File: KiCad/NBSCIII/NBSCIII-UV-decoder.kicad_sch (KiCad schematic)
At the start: 29 parts, among them U2 4053, U3 LM324N

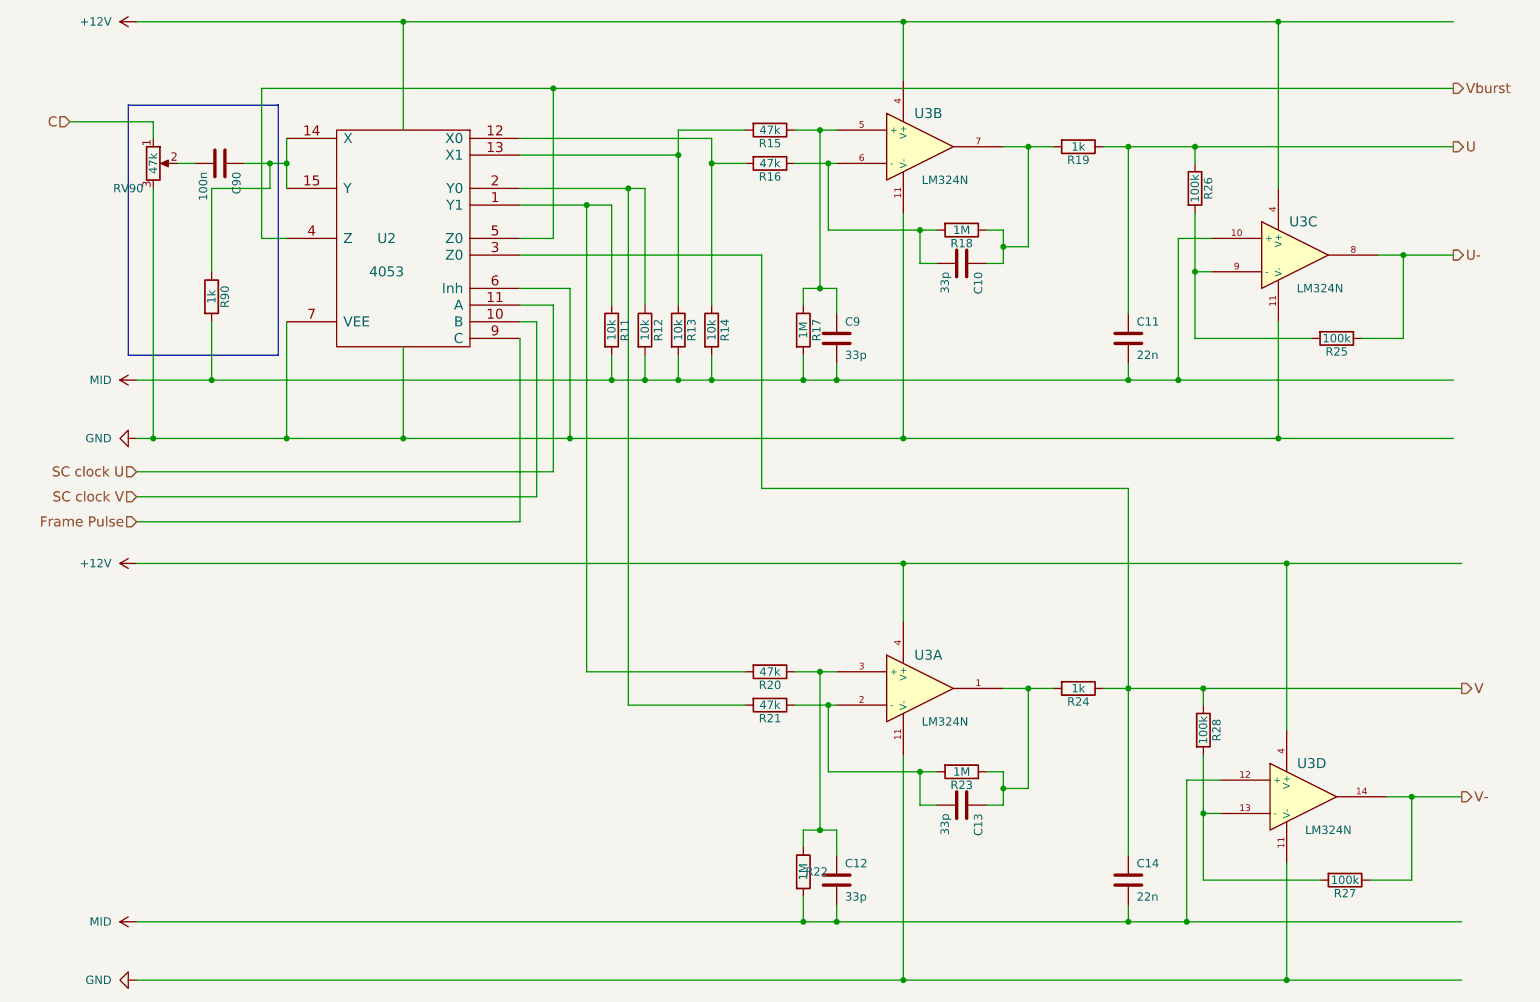
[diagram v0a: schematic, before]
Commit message: derescue 4053
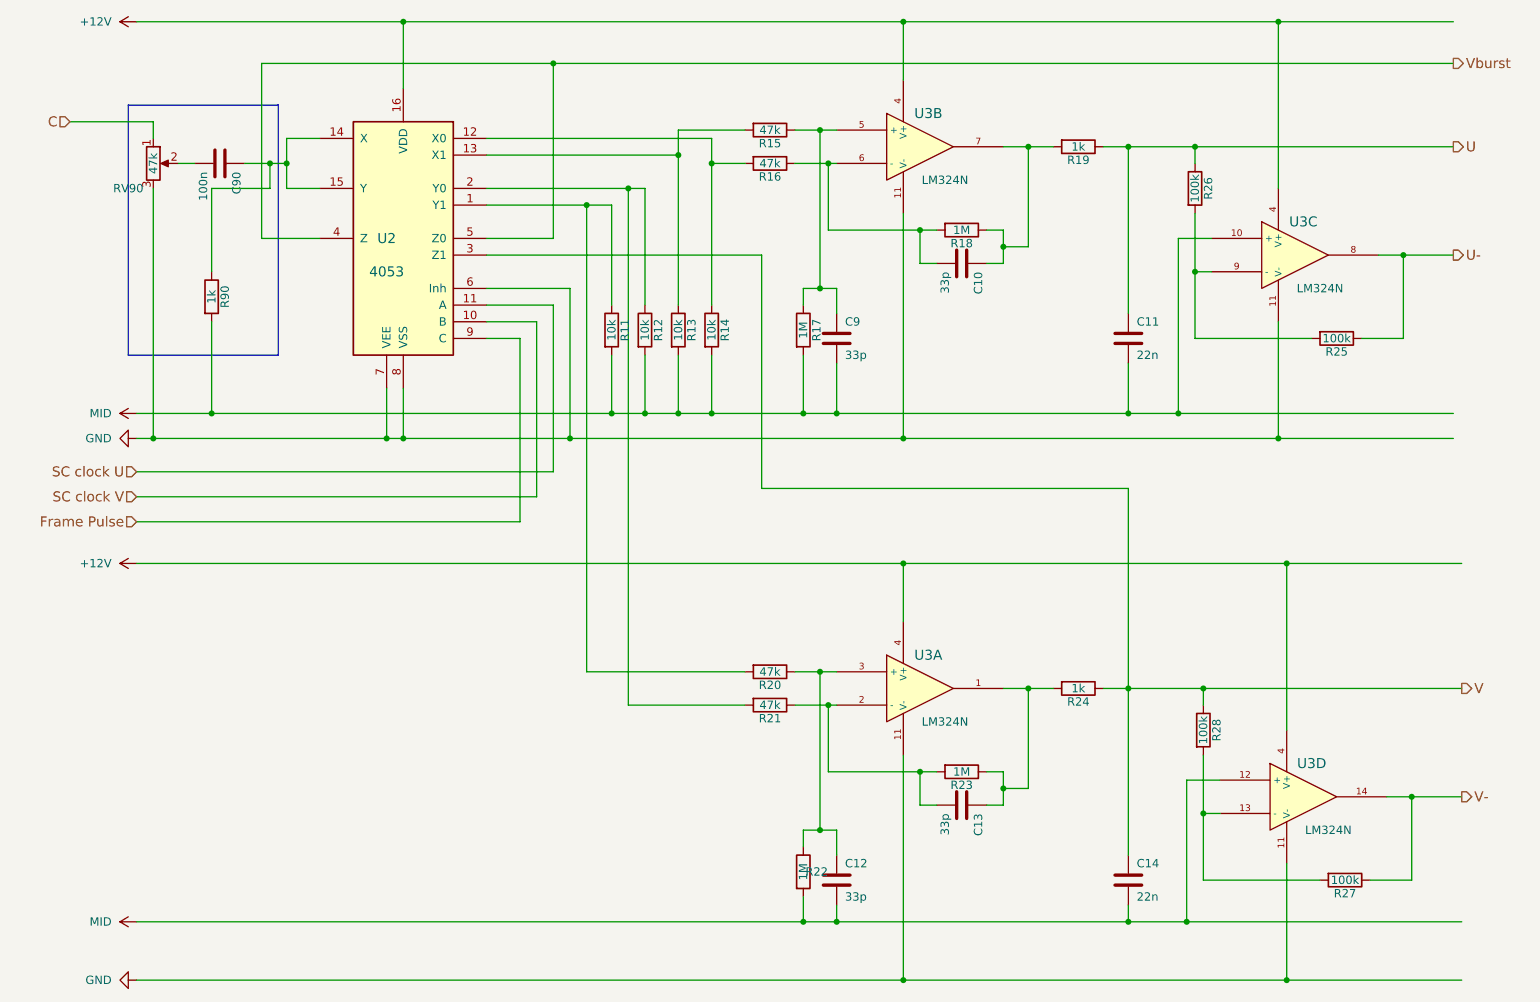
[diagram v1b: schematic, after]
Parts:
- U2: symbol NBSCIII-rescue:4053 -> 4xxx:4053
